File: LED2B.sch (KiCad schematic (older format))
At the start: 17 parts

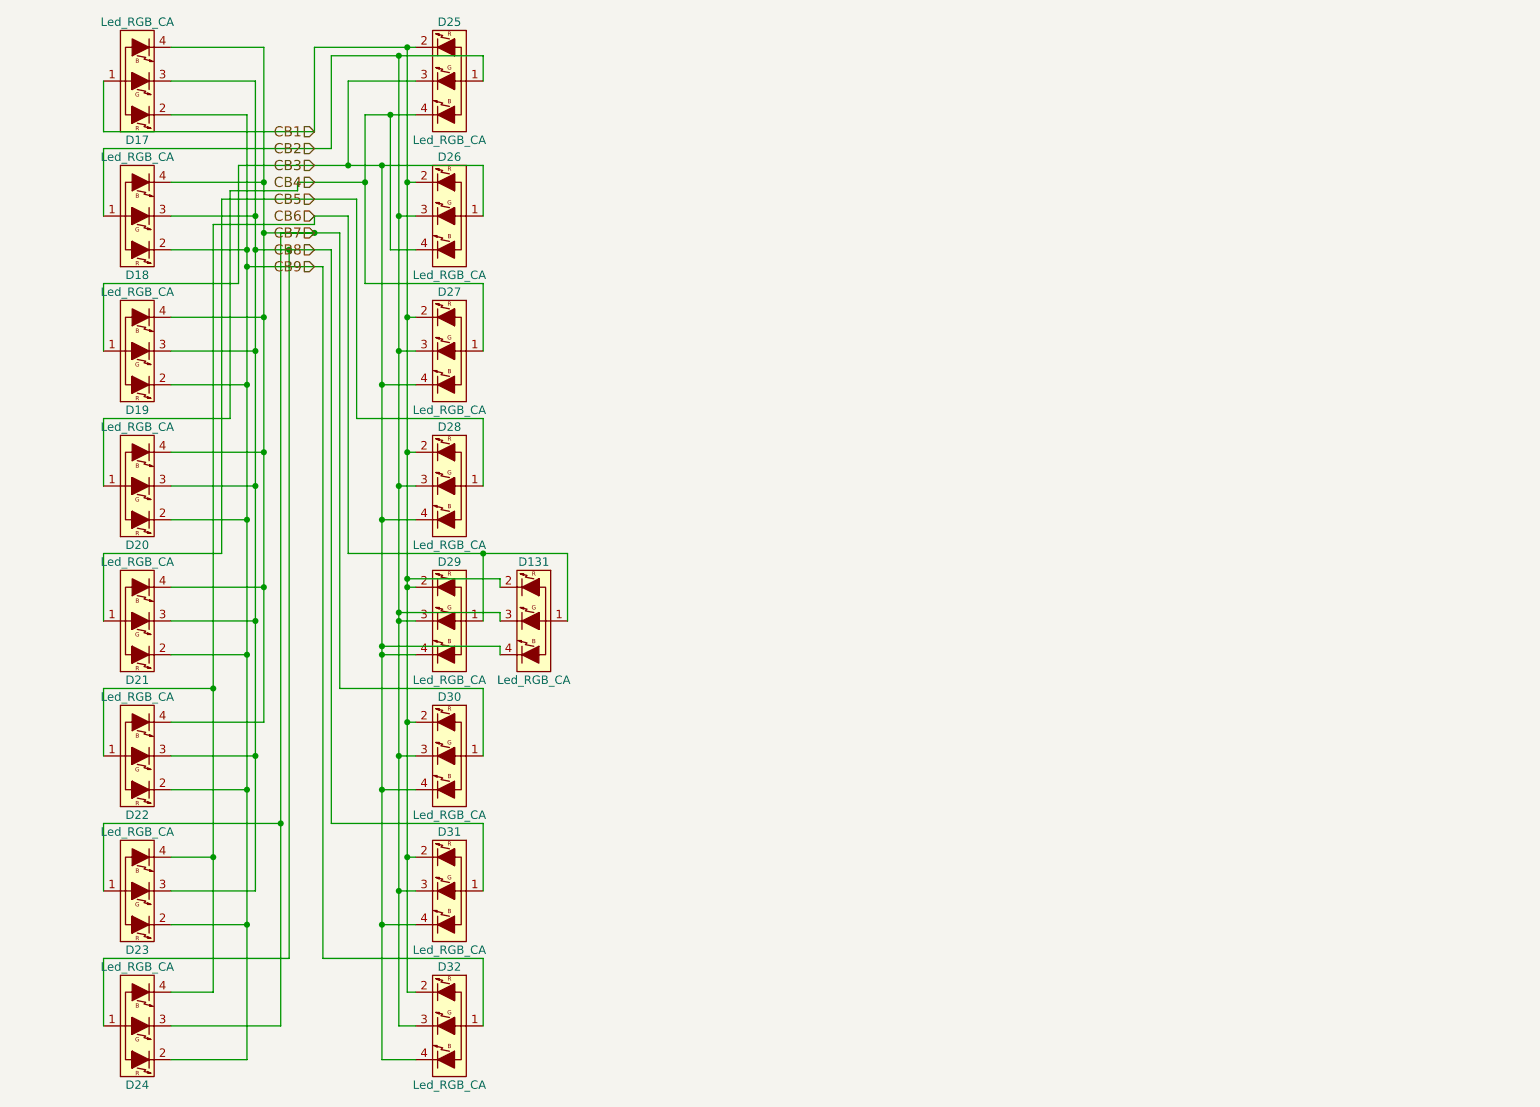
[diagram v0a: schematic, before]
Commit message: Clean up LED-Schematics
Luckily I didn't make any mistakes in the first run.
(Unless I made the same Mistake twice)
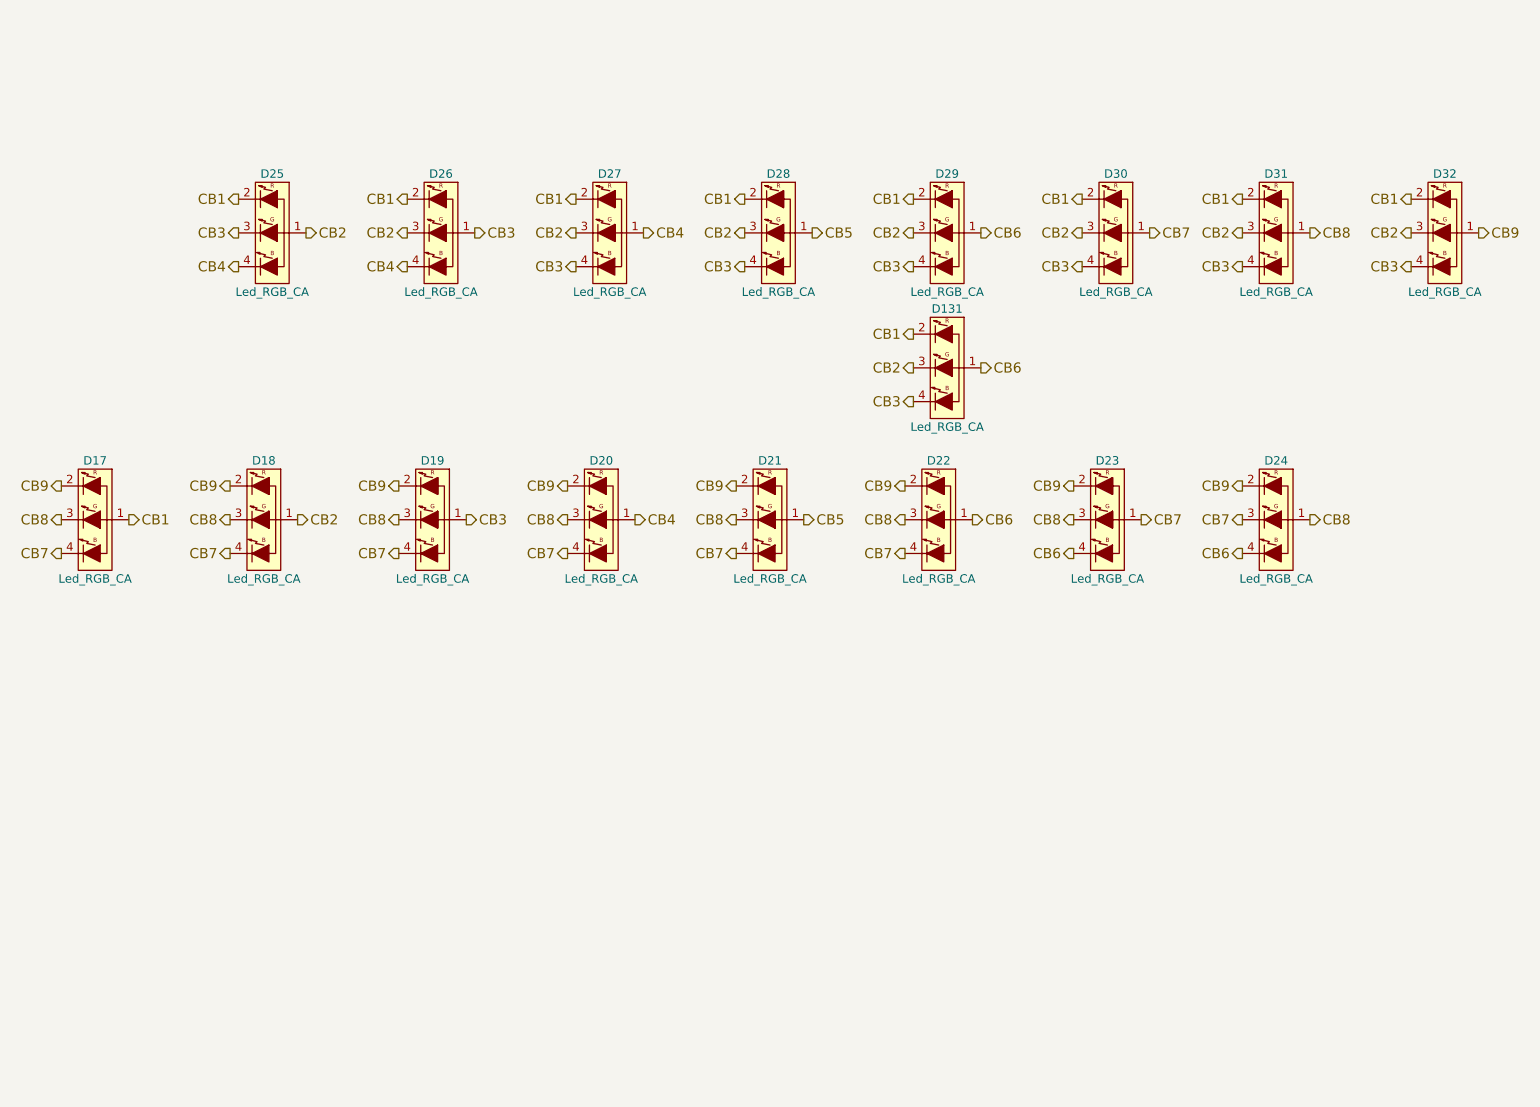
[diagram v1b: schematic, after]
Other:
- moved on the sheet: D131, D17, D18, D19, D20, D21, D22, D23, D24, D25, D26, D27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
